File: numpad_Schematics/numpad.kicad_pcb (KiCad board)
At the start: 11 copper layers, 75.4 x 104 mm, 44 parts, among them J1 Encoder input, J2 power module input, J3 Display, U1 ESP32-DEVKIT-V1 Matrix Handler, U2 BOB-12009

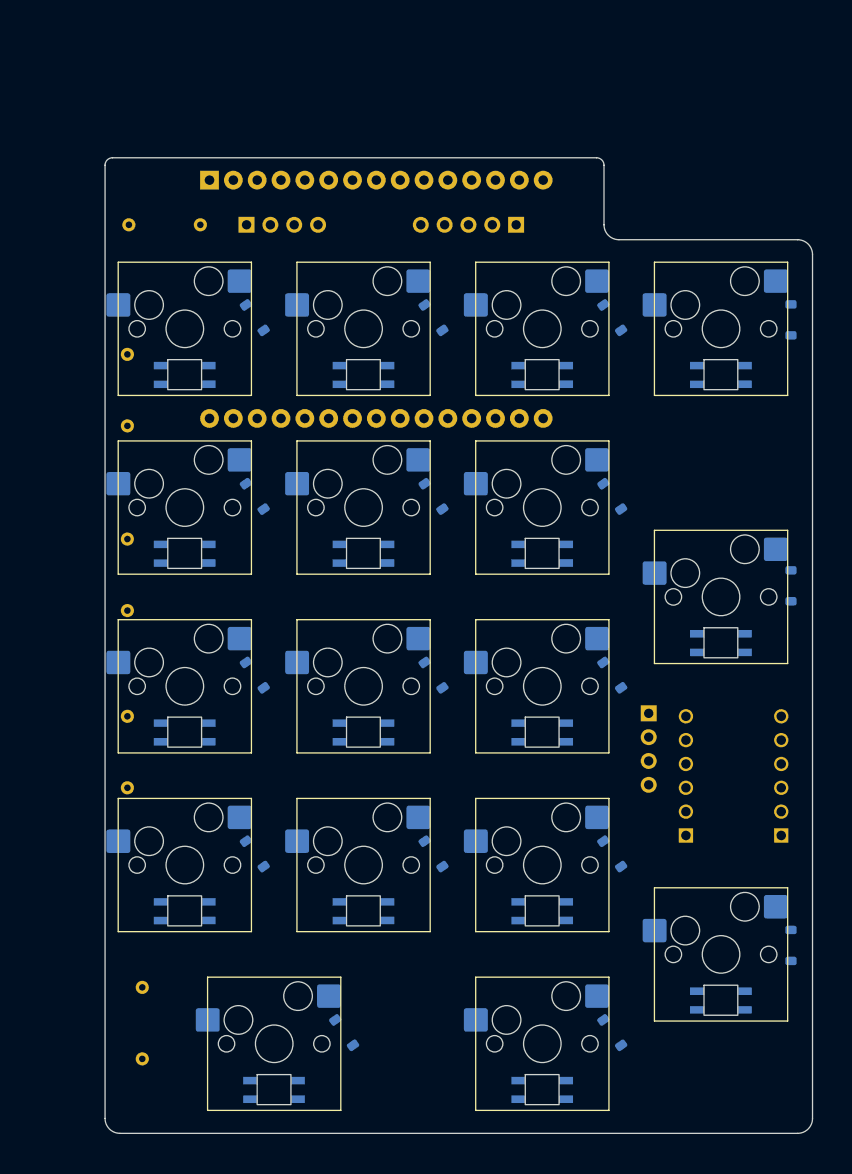
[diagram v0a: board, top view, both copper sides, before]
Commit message: case and pcb design
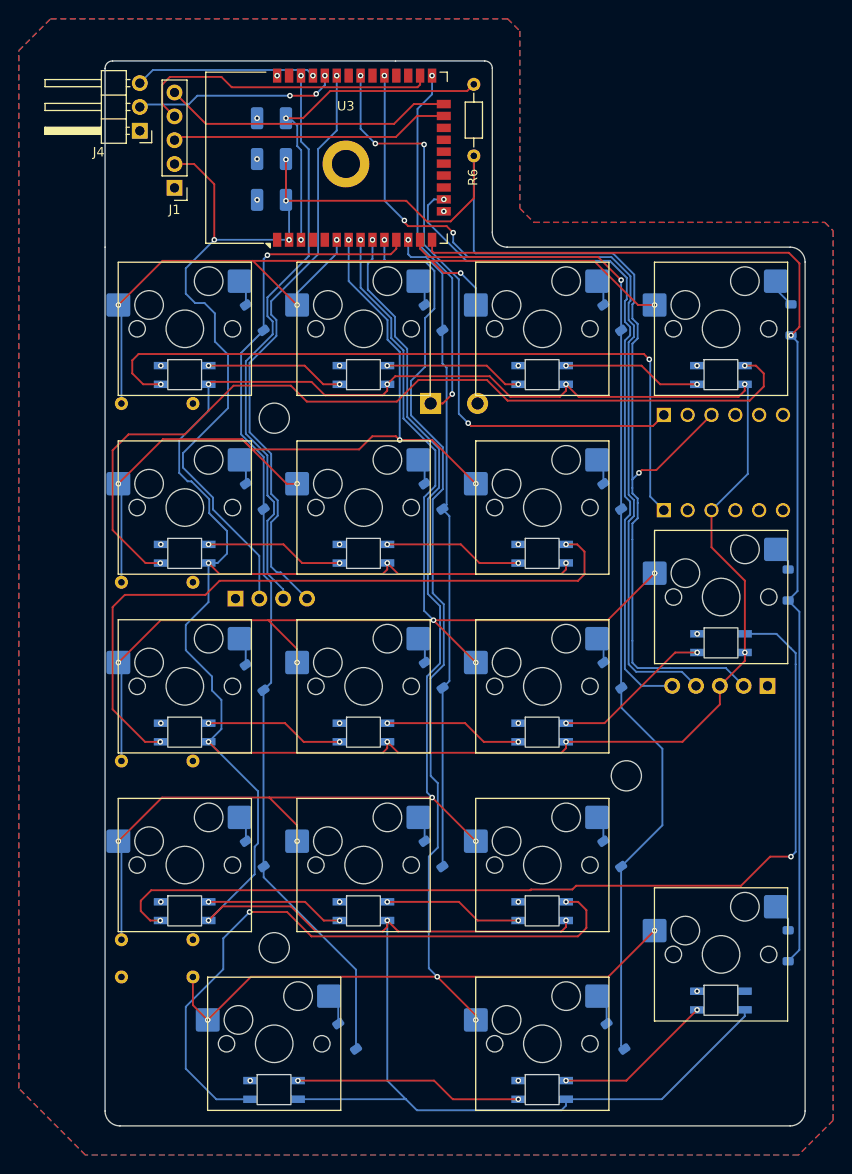
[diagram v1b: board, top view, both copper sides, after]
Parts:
- removed U1: ESP32-DEVKIT-V1 Matrix Handler, tigmitNIGHTLY:ESP32 Vroom Devkit V1 no holes
- added C1: 10uF, Capacitor_Tantalum_SMD:CP_EIA-3528-12_Kemet-T, B.Cu at (68.5, 40.2)
- added C2: 0.1uF, Capacitor_Tantalum_SMD:CP_EIA-3528-12_Kemet-T, B.Cu at (68.5, 35.9)
- added C3: tbd, Capacitor_Tantalum_SMD:CP_EIA-3528-12_Kemet-T, B.Cu at (68.5, 31.5)
- added J4: UART Download, Connector_PinHeader_2.54mm:PinHeader_1x03_P2.54mm_Horizontal, F.Cu at (54.5, 32.8)
- added R6: 10K, tigmitNIGHTLY:R_Axial_DIN0204_L3.6mm_D1.6mm_P7.62mm_Horizontal, F.Cu at (90.1, 35.5)
- added SW18: SW_Push, tigmitNIGHTLY:tigmit pushbutton, B.Cu at (85.0, 61.9)
- added U3: ESP32-WROOM-32, tigmitNIGHTLY:ESP32-WROOM-32 tigmit, F.Cu at (77.4, 35.7)
- D1, D10, D11, D12, D13, D14, D15, D16, D17, D2, D3, D4, D5, D6, D7, D8, D9: footprint TIGMIT_KEYBOARD_FOOTPRINTS:Diode_SOD-123 -> tigmitNIGHTLY:Diode_SOD-123
- J1: footprint TIGMIT_KEYBOARD_FOOTPRINTS:PinHeader_1x05_P2.54mm_Vertical -> tigmitNIGHTLY:PinHeader_1x05_P2.54mm_Vertical; moved to F.Cu
- J2: value power module input -> pwr input; footprint TIGMIT_KEYBOARD_FOOTPRINTS:PinHeader_1x04_P2.54mm_Vertical -> tigmitNIGHTLY:PinHeader_1x05_P2.54mm_Vertical
- J3: footprint TIGMIT_KEYBOARD_FOOTPRINTS:PinHeader_1x04_P2.54mm_Vertical -> tigmitNIGHTLY:PinHeader_1x04_P2.54mm_Vertical
- R1, R2, R3, R4, R5: footprint TIGMIT_KEYBOARD_FOOTPRINTS:R_Axial_DIN0204_L3.6mm_D1.6mm_P7.62mm_Horizontal -> tigmitNIGHTLY:R_Axial_DIN0204_L3.6mm_D1.6mm_P7.62mm_Horizontal
- SW1, SW10, SW11, SW12, SW13, SW14, SW15, SW16, SW17, SW2, SW3, SW4, SW5, SW6, SW7, SW8, SW9: footprint TIGMIT_KEYBOARD_FOOTPRINTS:hotswap socket with neopixel -> tigmitNIGHTLY:hotswap socket with neopixel
- U2: footprint TIGMIT_KEYBOARD_FOOTPRINTS:CONV_BOB-12009 -> tigmitNIGHTLY:CONV_BOB-12009
- moved D8 58.0 mm to (66.7, 91.1), turned to -55 degrees
- moved SW8 57.9 mm to (59.3, 92.0)
- moved SW15 48.6 mm to (68.8, 130.1)
- moved D15 48.3 mm to (76.6, 129.4), turned to -55 degrees
- moved J3 39.9 mm to (64.7, 82.7)
- moved J1 36.6 mm to (58.2, 38.9), turned to 180 degrees
- moved U2 33.4 mm to (116.7, 68.2), turned to -90 degrees
- moved D16 28.9 mm to (105.2, 129.3)
- moved SW16 28.6 mm to (97.4, 130.1)
- moved SW11 21.3 mm to (116.4, 82.5)
- moved SW17 21.3 mm to (116.4, 120.6)
- moved D11 21.1 mm to (123.6, 81.2), turned to -90 degrees
- moved D17 20.9 mm to (123.6, 119.7), turned to -90 degrees
- moved D10 19.1 mm to (104.9, 90.9)
- moved D9 19.1 mm to (85.8, 90.9)
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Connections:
- net NEOPIXEL5VData renamed NEOPIXEL5VData_KEYS
- J2 pad 1: batt_chargesense -> GND
- J2 pad 2: batt_voltage_Pin -> LV
- J2 pad 3: GND -> HV
- J2 pad 4: HV -> batt_chargesense
- J3 pad 1: SDA -> GND
- J3 pad 2: SCL -> LV
- J3 pad 3: LV -> SCL
- J3 pad 4: GND -> SDA
- R1 pad 1: Col2 -> Row0
- SW1 pad 1: Col2 -> Row0
- SW2 pad 1: Col2 -> Row0
- SW3 pad 1: Col2 -> Row0
- SW4 pad 1: Col2 -> Row0
- U2 pad LV1: NEOPIXEL_CONTROLL -> NEOPIXEL_CONTROLL_KEYS
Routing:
- net HV: track 0.00 -> 385.7 mm, vias 0 -> 14
- net LV: track 0.00 -> 201.0 mm, vias 0 -> 5
- net Row4: track 0.00 -> 151.3 mm, vias 0 -> 5
- net Row2: track 0.00 -> 128.6 mm, vias 0 -> 6
- net Row3: track 0.00 -> 123.1 mm, vias 0 -> 5
- net Col3: track 0.00 -> 117.3 mm, vias 0 -> 1
- net Col2: track 0.00 -> 109.5 mm, vias 0 -> 1
- net Col0: track 0.00 -> 106.5 mm, vias 0 -> 1
- net Net-(SW11-DO): track 0.00 -> 103.0 mm, vias 0 -> 2
- net Row0: track 0.00 -> 94.7 mm, vias 0 -> 5
- net Net-(SW4-DO): track 0.00 -> 94.3 mm, vias 0 -> 2
- net batt_chargesense: track 0.00 -> 94.1 mm, vias 0 -> 3
- net Row1: track 0.00 -> 85.3 mm, vias 0 -> 5
- net NEOPIXEL5VData_KEYS: track 0.00 -> 77.3 mm, vias 0 -> 2
- net batt_voltage_Pin: track 0.00 -> 75.9 mm, vias 0 -> 1
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- added copper zone on B.Cu, net GND
- added copper zone on F.Cu, net GND
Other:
- board size 75.4 x 104 mm -> 74.6 x 113.5 mm
- board text added: "GND |3.3V | 5V | bSense | vBatt"
